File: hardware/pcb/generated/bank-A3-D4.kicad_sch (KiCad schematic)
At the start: 34 parts, among them U22 SK9822-EC20, U23 SK9822-EC20, U24 SK9822-EC20, U25 SK9822-EC20, U3 TCA9554DWR, U34 SK9822-EC20, U35 SK9822-EC20, U36 SK9822-EC20, U37 SK9822-EC20

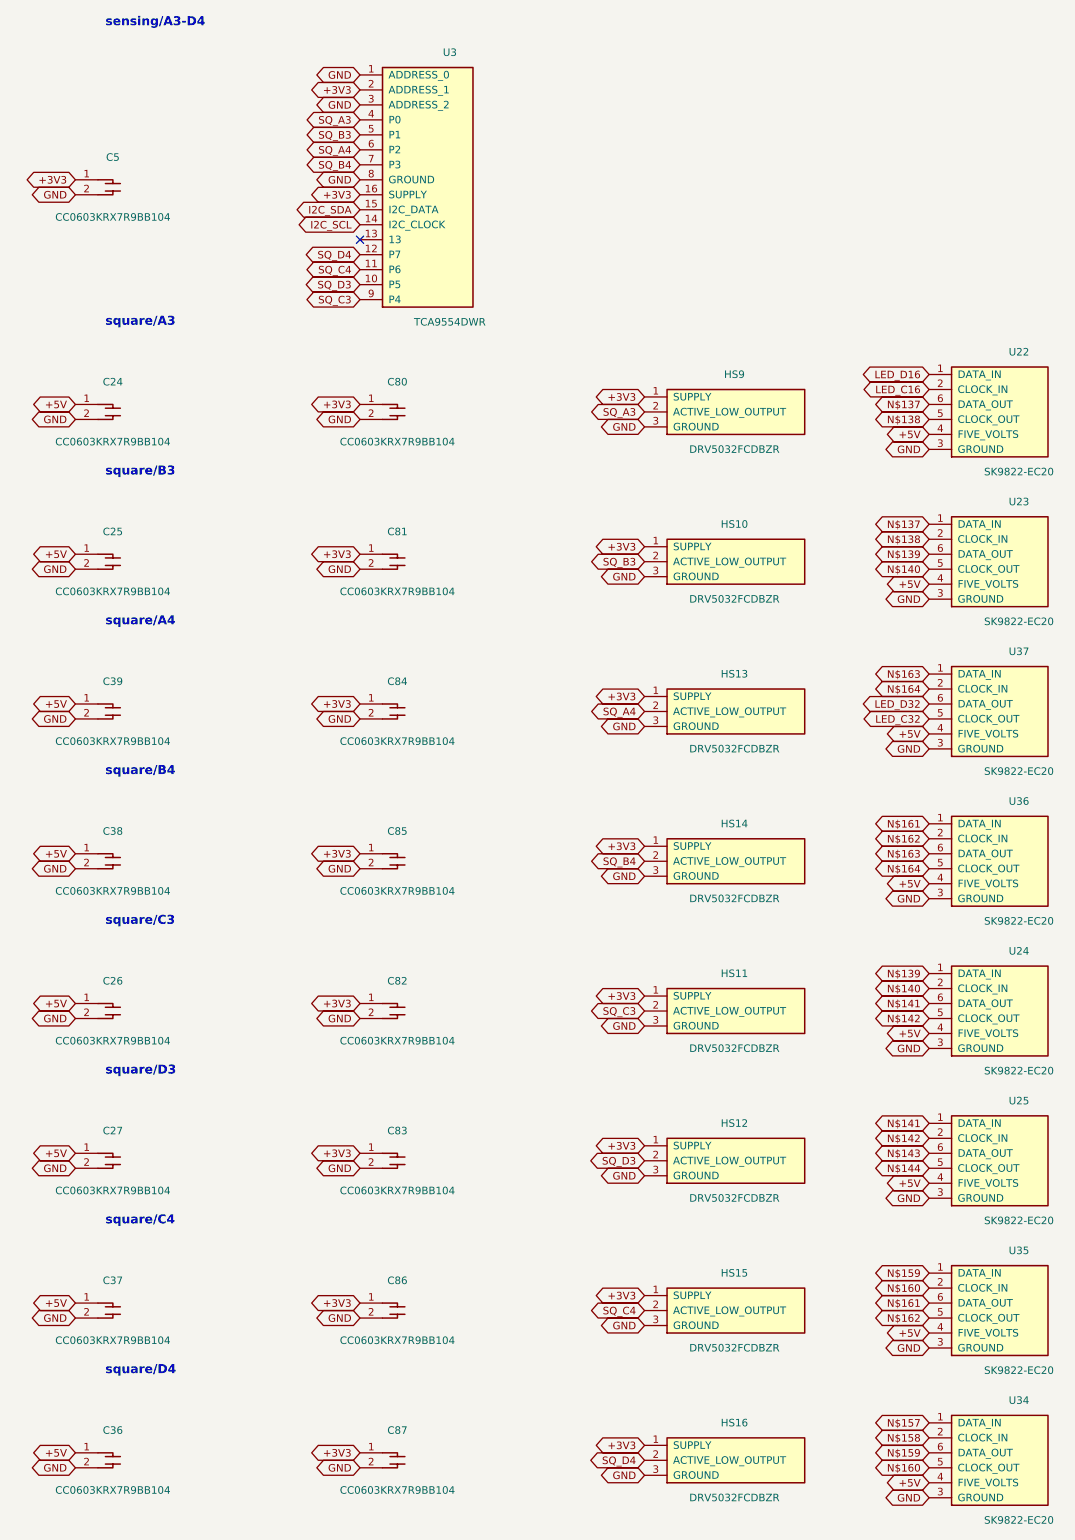
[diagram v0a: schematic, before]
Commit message: chore(pcb): regenerate KiCad, SPICE and review output
Generated by `just pcb` from the committed definition; not hand-edited.
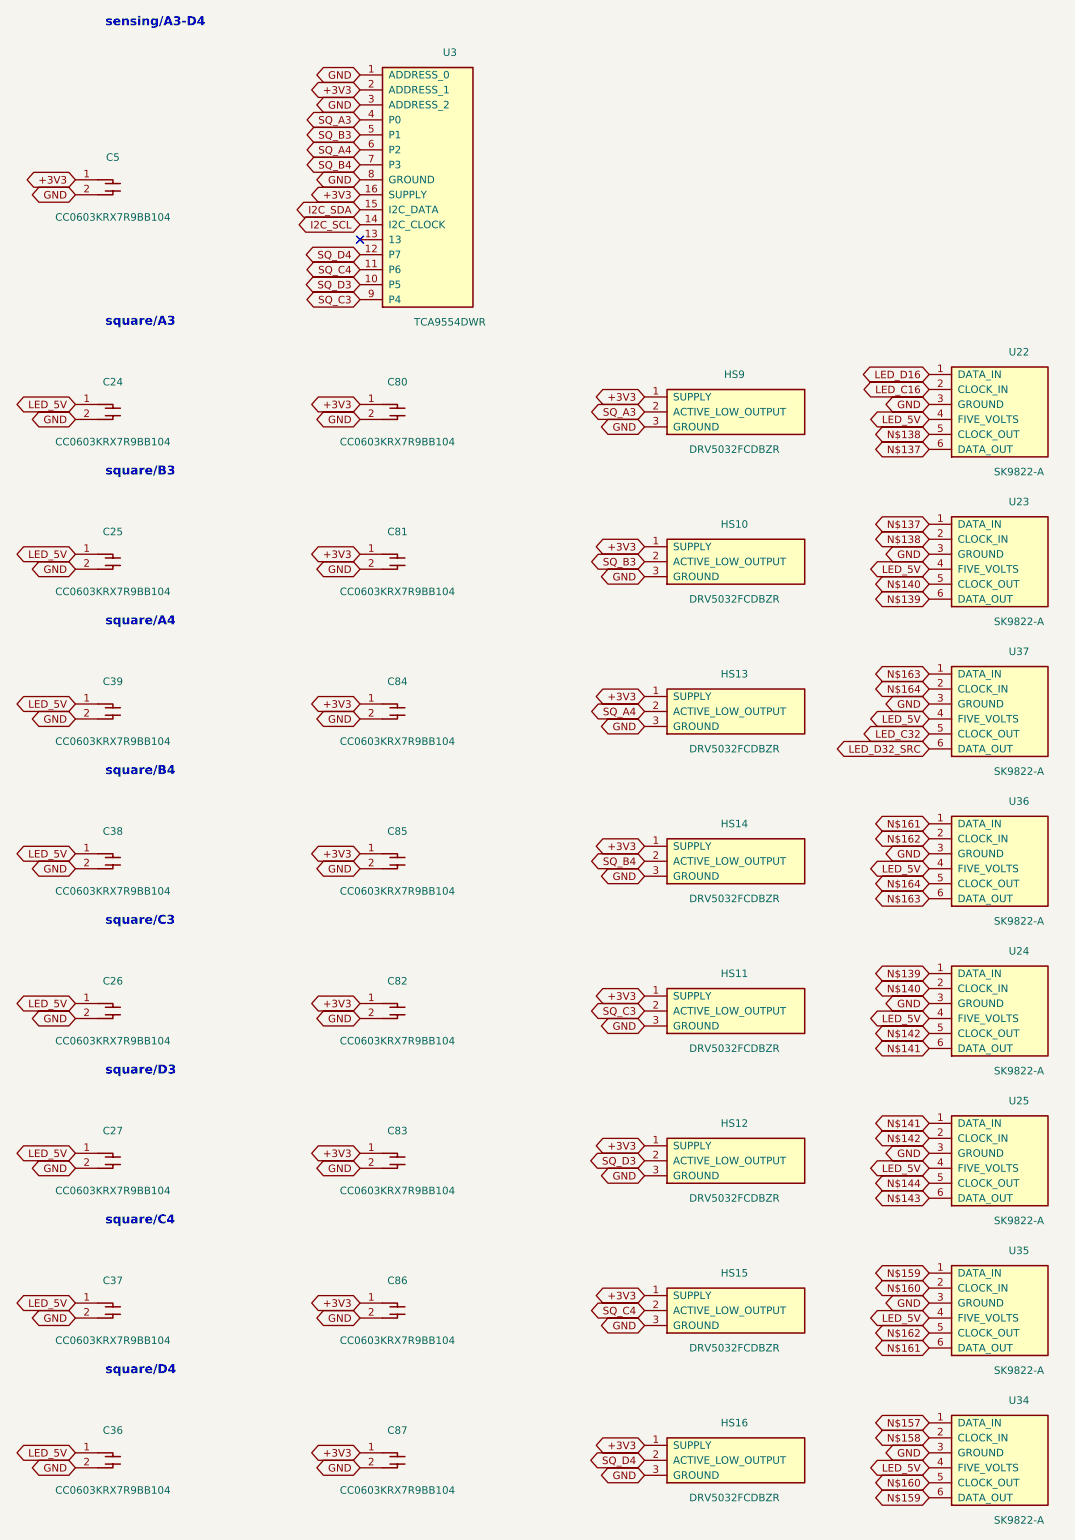
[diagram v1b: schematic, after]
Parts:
- U22, U23, U24, U25, U34, U35, U36, U37: value SK9822-EC20 -> SK9822-A
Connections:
- net +5V renamed LED_5V
- net LED_D32 renamed LED_D32_SRC
